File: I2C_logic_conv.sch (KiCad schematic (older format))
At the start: 5 parts, among them Q1 BSS138PS

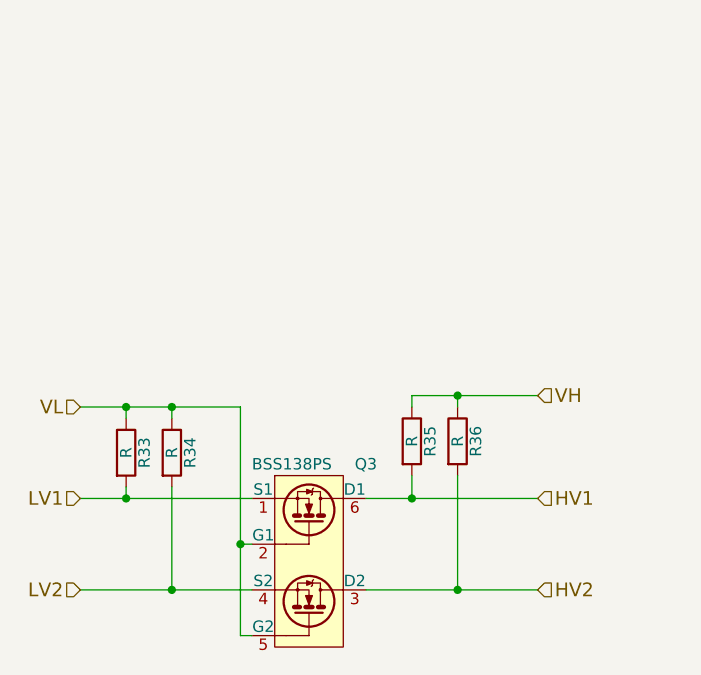
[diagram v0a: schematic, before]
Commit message: 進捗
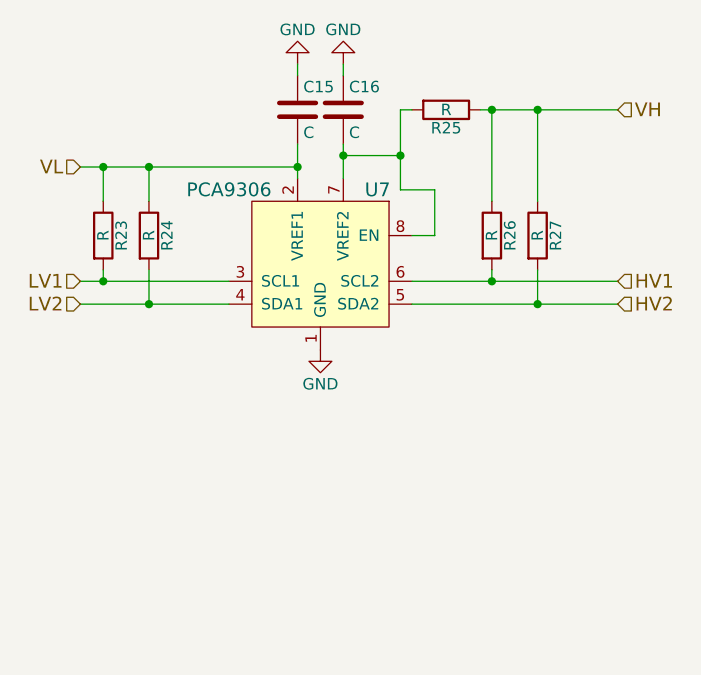
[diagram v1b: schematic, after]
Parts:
- removed Q1: BSS138PS, SMD_Packages:SOT363, symbol BSS138PS
- added C6, C7: C, Capacitors_SMD:C_0603, symbol C
- added R14: R, Resistors_SMD:R_0603, symbol R
- added U4: PCA9306, Housings_SSOP:MSOP-8_3x3mm_Pitch0.65mm, symbol PCA9306
- renumbered R24 to R12, R25 to R13, R26 to R15, R27 to R16
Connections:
- net HV1: now also U4.6 (SCL2)
- net HV2: now also U4.5 (SDA2)
- net LV1: now also U4.3 (SCL1)
- net LV2: now also U4.4 (SDA1)
- net VH: now also R14.1
- net VL: now also C6.2, U4.2 (VREF1)
- new net: C7.2, R14.2, U4.7 (VREF2), U4.8 (EN)
- new net GND: C6.1, C7.1, U4.1 (GND)
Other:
- moved on the sheet: R23, R24, R26, R27
